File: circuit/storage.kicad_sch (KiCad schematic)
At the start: 23 parts, among them J16 Fortuna programmer, J17 Port A, J23 Port B, J24 Port C, J3 SDCard, J36 Port G, U19 4013, U3 ATmega328-P, Y1 16.5 Mhz

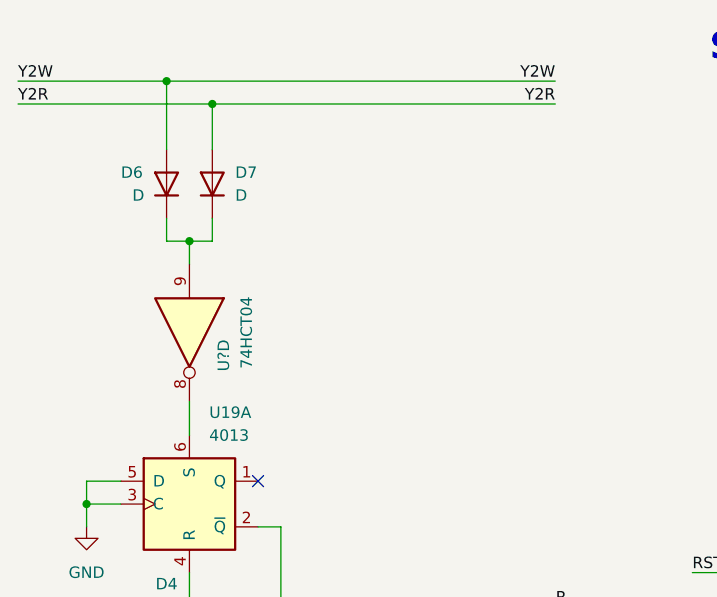
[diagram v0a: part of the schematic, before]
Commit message: .
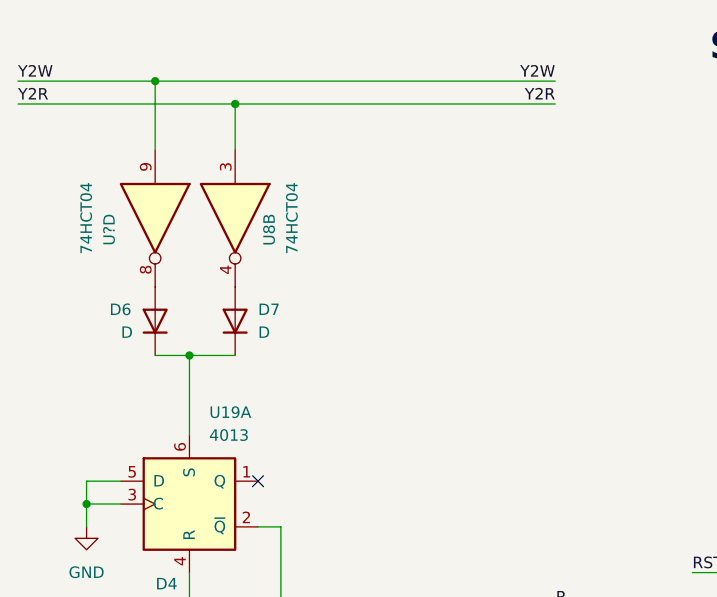
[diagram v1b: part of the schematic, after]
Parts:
- added U8: 74HCT04, symbol 74xx:74HCT04
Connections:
- net Y2R: now also U8.3; no longer D7.2 (A)
- net Y2W: now also U?.9; no longer D6.2 (A)
- net at U19.6 (S): now also D6.1 (K), D7.1 (K); no longer U?.8
- new net: D7.2 (A), U8.4
- new net: D6.2 (A), U?.8
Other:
- moved on the sheet: D6, D7, U?D
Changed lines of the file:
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@@
   (junction (at 142.24 59.69) (diameter 0) (color 0 0 0 0)
   )
+  (junction (at 35.56 53.34) (diameter 0) (color 0 0 0 0)
+  )
   (junction (at 53.34 125.73) (diameter 0) (color 0 0 0 0)
   )
@@
   (junction (at 132.08 59.69) (diameter 0) (color 0 0 0 0)
   )
-  (junction (at 35.56 40.64) (diameter 0) (color 0 0 0 0)
-  )
-  (junction (at 33.02 22.86) (diameter 0) (color 0 0 0 0)
-  )
-  (junction (at 38.1 25.4) (diameter 0) (color 0 0 0 0)
+  (junction (at 31.75 22.86) (diameter 0) (color 0 0 0 0)
+  )
+  (junction (at 40.64 25.4) (diameter 0) (color 0 0 0 0)
   )
   (no_connect (at 167.64 67.31))
@@
     (stroke (width 0) (type default))
   )
-  (wire (pts (xy 38.1 38.1) (xy 38.1 40.64))
-    (stroke (width 0) (type default))
-  )
   (wire (pts (xy 218.44 67.945) (xy 229.235 67.945))
     (stroke (width 0) (type default))
@@
     (stroke (width 0) (type default))
   )
-  (wire (pts (xy 38.1 25.4) (xy 76.2 25.4))
+  (wire (pts (xy 16.51 25.4) (xy 40.64 25.4))
     (stroke (width 0) (type default))
   )
@@
     (stroke (width 0) (type default))
   )
-  (wire (pts (xy 16.51 25.4) (xy 38.1 25.4))
-    (stroke (width 0) (type default))
-  )
   (wire (pts (xy 142.24 59.69) (xy 139.7 59.69))
     (stroke (width 0) (type default))
@@
     (stroke (width 0) (type default))
   )
-  (wire (pts (xy 33.02 38.1) (xy 33.02 40.64))
-    (stroke (width 0) (type default))
-  )
   (wire (pts (xy 256.54 34.29) (xy 256.54 43.18))
     (stroke (width 0) (type default))
@@
     (stroke (width 0) (type default))
   )
-  (wire (pts (xy 35.56 58.42) (xy 35.56 62.23))
+  (wire (pts (xy 35.56 53.34) (xy 35.56 62.23))
     (stroke (width 0) (type default))
   )
@@
     (stroke (width 0) (type default))
   )
+  (wire (pts (xy 40.64 25.4) (xy 76.2 25.4))
+    (stroke (width 0) (type default))
+  )
   (wire (pts (xy 147.32 57.15) (xy 147.32 59.69))
     (stroke (width 0) (type default))
@@
     (stroke (width 0) (type default))
   )
-  (wire (pts (xy 16.51 22.86) (xy 33.02 22.86))
+  (wire (pts (xy 16.51 22.86) (xy 31.75 22.86))
     (stroke (width 0) (type default))
   )
@@
     (stroke (width 0) (type default))
   )
-  (wire (pts (xy 38.1 40.64) (xy 35.56 40.64))
-    (stroke (width 0) (type default))
-  )
   (wire (pts (xy 218.44 96.52) (xy 229.235 96.52))
     (stroke (width 0) (type default))
@@
     (stroke (width 0) (type default))
   )
-  (wire (pts (xy 33.02 22.86) (xy 76.2 22.86))
-    (stroke (width 0) (type default))
-  )
-  (wire (pts (xy 33.02 22.86) (xy 33.02 30.48))
+  (wire (pts (xy 31.75 22.86) (xy 76.2 22.86))
+    (stroke (width 0) (type default))
+  )
+  (wire (pts (xy 31.75 22.86) (xy 31.75 30.48))
     (stroke (width 0) (type default))
   )
@@
     (stroke (width 0) (type default))
   )
+  (wire (pts (xy 35.56 53.34) (xy 40.64 53.34))
+    (stroke (width 0) (type default))
+  )
   (wire (pts (xy 218.44 65.405) (xy 229.235 65.405))
     (stroke (width 0) (type default))
@@
     (stroke (width 0) (type default))
   )
-  (wire (pts (xy 33.02 40.64) (xy 35.56 40.64))
-    (stroke (width 0) (type default))
-  )
   (wire (pts (xy 271.145 75.565) (xy 260.35 75.565))
     (stroke (width 0) (type default))
@@
     (stroke (width 0) (type default))
   )
+  (wire (pts (xy 31.75 53.34) (xy 35.56 53.34))
+    (stroke (width 0) (type default))
+  )
   (wire (pts (xy 156.21 49.53) (xy 167.64 49.53))
     (stroke (width 0) (type default))
@@
     (stroke (width 0) (type default))
   )
-  (wire (pts (xy 38.1 25.4) (xy 38.1 30.48))
-    (stroke (width 0) (type default))
-  )
   (wire (pts (xy 55.88 138.43) (xy 55.88 140.97))
     (stroke (width 0) (type default))
@@
     (stroke (width 0) (type default))
   )
-  (wire (pts (xy 35.56 40.64) (xy 35.56 43.18))
+  (wire (pts (xy 40.64 25.4) (xy 40.64 30.48))
     (stroke (width 0) (type default))
   )
@@
     )
   )
-  (symbol (lib_id "Device:D") (at 38.1 34.29 90) (unit 1)
-    (in_bom yes) (on_board yes) (dnp no) (fields_autoplaced)
-    (property "Reference" "D7" (at 40.64 33.02 90)
+  (symbol (lib_id "Device:D") (at 40.64 49.53 90) (unit 1)
+    (in_bom yes) (on_board yes) (dnp no) (fields_autoplaced)
+    (property "Reference" "D7" (at 43.18 48.26 90)
       (effects (font (size 1.27 1.27)) (justify right))
     )
-    (property "Value" "D" (at 40.64 35.56 90)
+    (property "Value" "D" (at 43.18 50.8 90)
       (effects (font (size 1.27 1.27)) (justify right))
     )
-    (property "Footprint" "" (at 38.1 34.29 0)
-      (effects (font (size 1.27 1.27)) hide)
-    )
-    (property "Datasheet" "~" (at 38.1 34.29 0)
-      (effects (font (size 1.27 1.27)) hide)
-    )
-    (property "Sim.Device" "D" (at 38.1 34.29 0)
-      (effects (font (size 1.27 1.27)) hide)
-    )
-    (property "Sim.Pins" "1=K 2=A" (at 38.1 34.29 0)
+    (property "Footprint" "" (at 40.64 49.53 0)
+      (effects (font (size 1.27 1.27)) hide)
+    )
+    (property "Datasheet" "~" (at 40.64 49.53 0)
+      (effects (font (size 1.27 1.27)) hide)
+    )
+    (property "Sim.Device" "D" (at 40.64 49.53 0)
+      (effects (font (size 1.27 1.27)) hide)
+    )
+    (property "Sim.Pins" "1=K 2=A" (at 40.64 49.53 0)
       (effects (font (size 1.27 1.27)) hide)
     )
@@
     )
   )
-  (symbol (lib_id "Device:D") (at 33.02 34.29 90) (unit 1)
+  (symbol (lib_id "Device:D") (at 31.75 49.53 90) (unit 1)
     (in_bom yes) (on_board yes) (dnp no)
-    (property "Reference" "D6" (at 27.94 33.02 90)
+    (property "Reference" "D6" (at 26.67 48.26 90)
       (effects (font (size 1.27 1.27)) (justify right))
     )
-    (property "Value" "D" (at 29.21 35.56 90)
+    (property "Value" "D" (at 27.94 50.8 90)
       (effects (font (size 1.27 1.27)) (justify right))
     )
-    (property "Footprint" "" (at 33.02 34.29 0)
-      (effects (font (size 1.27 1.27)) hide)
-    )
-    (property "Datasheet" "~" (at 33.02 34.29 0)
-      (effects (font (size 1.27 1.27)) hide)
-    )
-    (property "Sim.Device" "D" (at 33.02 34.29 0)
-      (effects (font (size 1.27 1.27)) hide)
-    )
-    (property "Sim.Pins" "1=K 2=A" (at 33.02 34.29 0)
+    (property "Footprint" "" (at 31.75 49.53 0)
+      (effects (font (size 1.27 1.27)) hide)
+    )
+    (property "Datasheet" "~" (at 31.75 49.53 0)
+      (effects (font (size 1.27 1.27)) hide)
+    )
+    (property "Sim.Device" "D" (at 31.75 49.53 0)
+      (effects (font (size 1.27 1.27)) hide)
+    )
+    (property "Sim.Pins" "1=K 2=A" (at 31.75 49.53 0)
       (effects (font (size 1.27 1.27)) hide)
     )
@@
     )
   )
-  (symbol (lib_id "74xx:74HCT04") (at 35.56 50.8 270) (unit 4)
+  (symbol (lib_id "74xx:74HCT04") (at 40.64 38.1 270) (unit 2)
     (in_bom yes) (on_board yes) (dnp no)
-    (property "Reference" "U?" (at 39.37 53.34 0)
-      (effects (font (size 1.27 1.27)))
-    )
-    (property "Value" "74HCT04" (at 41.91 50.8 0)
-      (effects (font (size 1.27 1.27)))
-    )
-    (property "Footprint" "" (at 35.56 50.8 0)
-      (effects (font (size 1.27 1.27)) hide)
-    )
-    (property "Datasheet" "https://assets.nexperia.com/documents/data-sheet/74HC_HCT04.pdf" (at 35.56 50.8 0)
-      (effects (font (size 1.27 1.27)) hide)
-    )
+    (property "Reference" "U8" (at 44.45 39.37 0)
+      (effects (font (size 1.27 1.27)))
+    )
+    (property "Value" "74HCT04" (at 46.99 38.1 0)
+      (effects (font (size 1.27 1.27)))
+    )
+    (property "Footprint" "" (at 40.64 38.1 0)
+      (effects (font (size 1.27 1.27)) hide)
+    )
+    (property "Datasheet" "https://assets.nexperia.com/documents/data-sheet/74HC_HCT04.pdf" (at 40.64 38.1 0)
+      (effects (font (size 1.27 1.27)) hide)
+    )
+    (pin "1")
+    (pin "2")
+    (pin "3")
+    (pin "4")
+    (pin "5")
+    (pin "6")
+    (pin "8")
+    (pin "9")
+    (pin "10")
+    (pin "11")
+    (pin "12")
+    (pin "13")
+    (pin "14")
+    (pin "7")
+    (instances
+      (project "fortuna-box"
+        (path "/0e4c4e8a-78e0-4f49-88dc-754c12656209/0ad0c907-f2a9-47ff-aff1-7aaecbdef7ee"
+          (reference "U8") (unit 2)
+        )
+      )
+    )
+  )
+  (symbol (lib_id "74xx:74HCT04") (at 31.75 38.1 270) (unit 4)
+    (in_bom yes) (on_board yes) (dnp no)
+    (property "Reference" "U?" (at 26.67 39.37 0)
+      (effects (font (size 1.27 1.27)))
+    )
+    (property "Value" "74HCT04" (at 24.13 38.1 0)
+      (effects (font (size 1.27 1.27)))
+    )
+    (property "Footprint" "" (at 31.75 38.1 0)
+      (effects (font (size 1.27 1.27)) hide)
+    )
+    (property "Datasheet" "https://assets.nexperia.com/documents/data-sheet/74HC_HCT04.pdf" (at 31.75 38.1 0)
+      (effects (font (size 1.27 1.27)) hide)
+    )
